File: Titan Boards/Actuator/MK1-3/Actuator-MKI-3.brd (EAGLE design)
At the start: 101.6 x 55.9 mm, 56 parts, among them U1 DRV8816PWPR, U2 MBRB2060CTT4G, U3 MBRB2060CTT4G, U4 MBRB2060CTT4G, U5 MBRB2060CTT4G, U6 MBRB2060CTT4G, U7 MBRB2060CTT4G

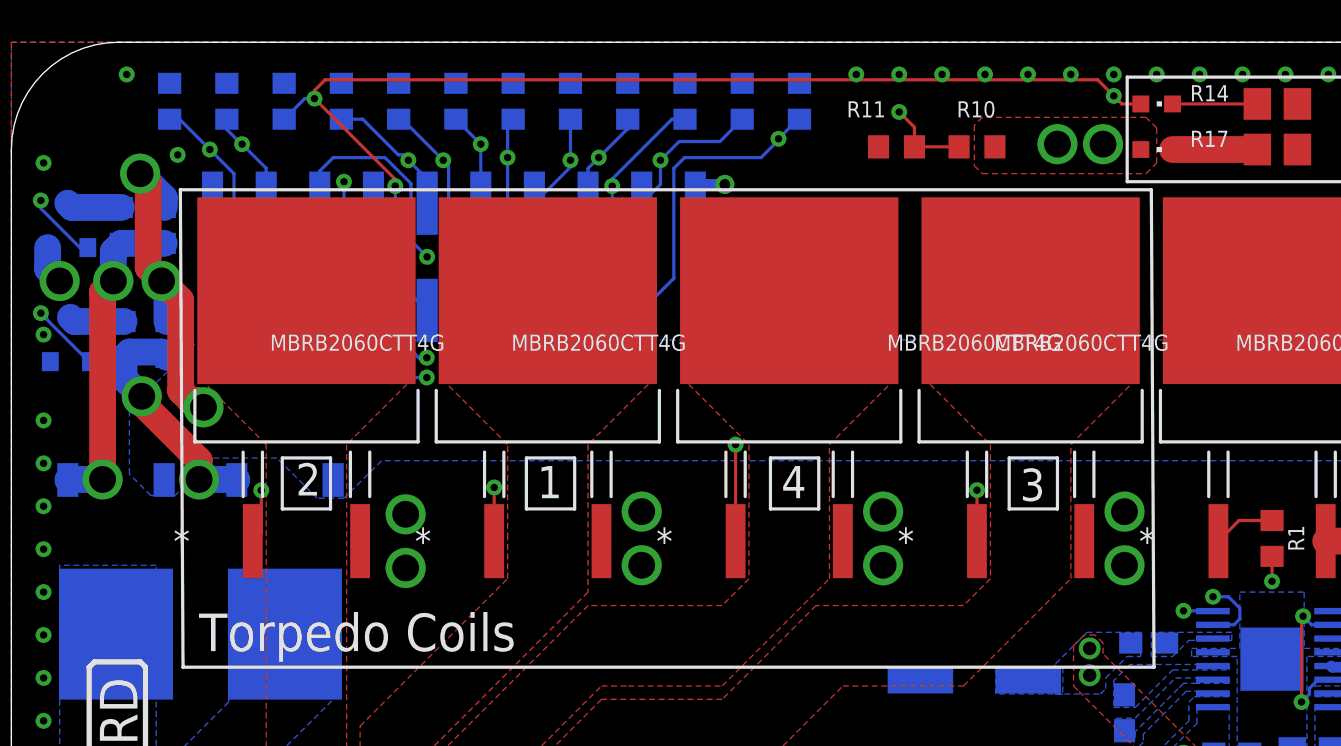
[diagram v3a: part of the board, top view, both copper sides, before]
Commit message: Tempest Actuator Updates
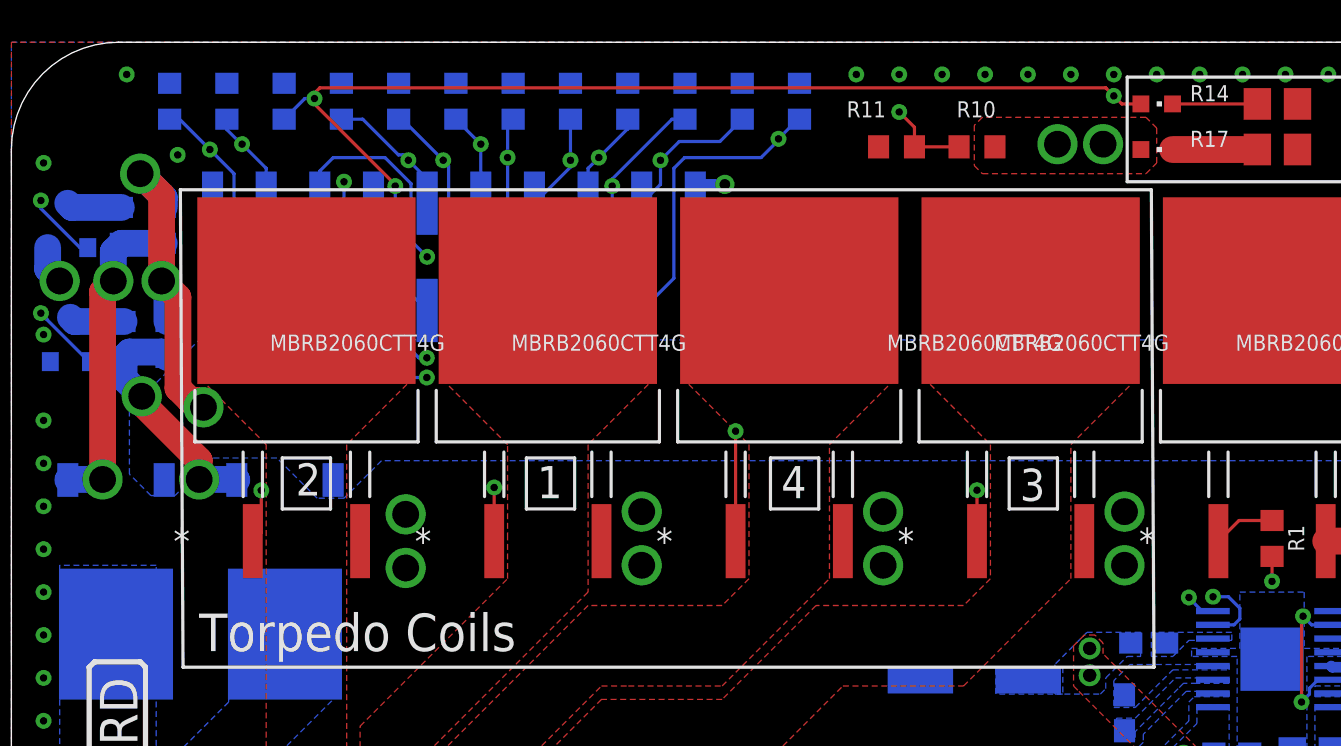
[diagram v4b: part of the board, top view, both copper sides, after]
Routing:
- net PWM_DRIVER1: track 77.5 -> 80.4 mm
- net VPROPI: track 59.1 -> 59.8 mm

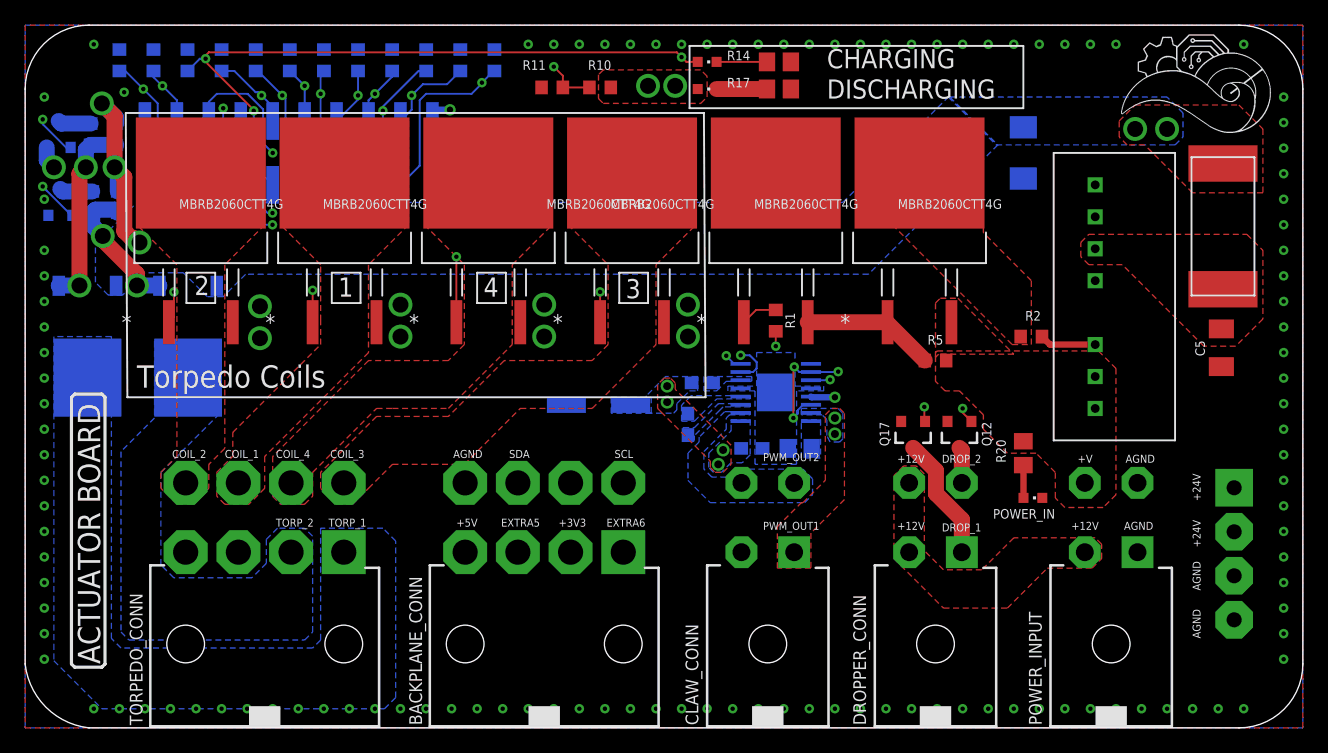
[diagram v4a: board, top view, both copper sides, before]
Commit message: Tempest Actuator Board Review Revisions
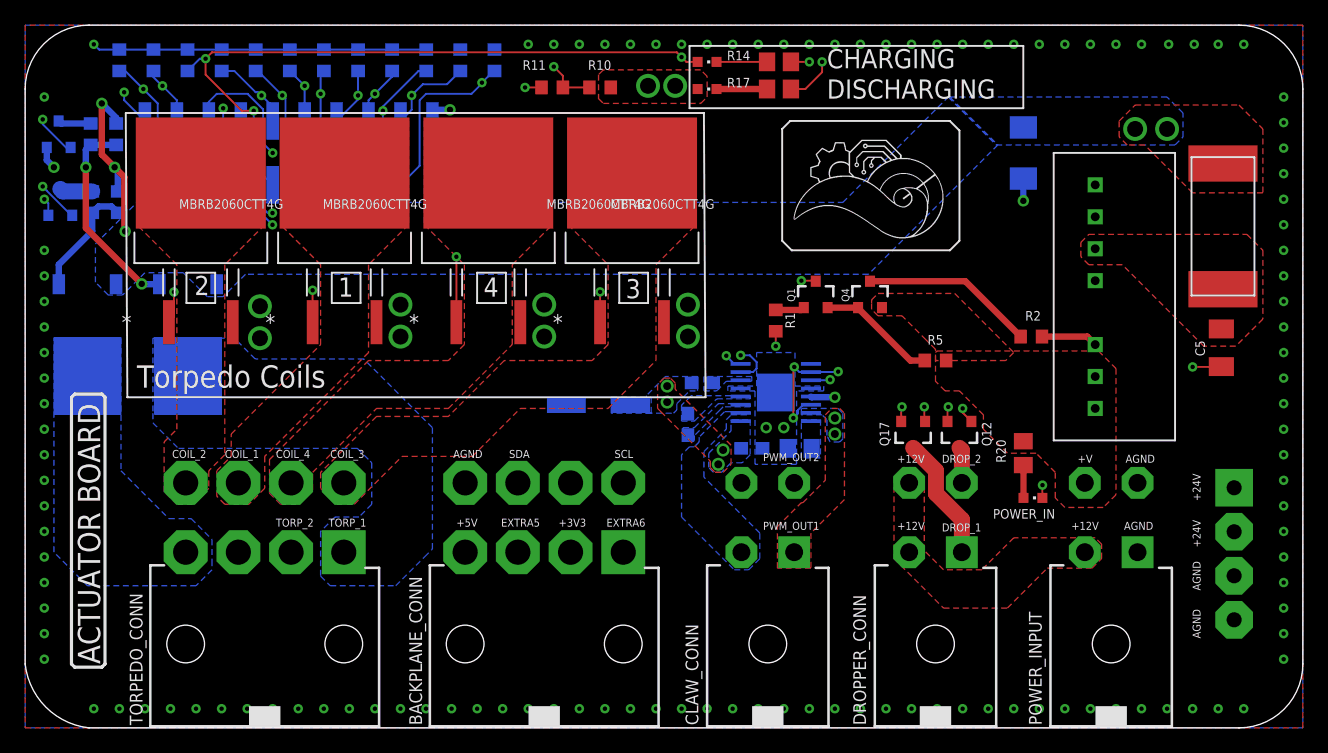
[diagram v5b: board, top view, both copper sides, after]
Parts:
- removed U6, U7: MBRB2060CTT4G, DPAK2:D2PAK3-4_9P65X10P29_ONS
- added Q1, Q4: (no value), SparkFun-DiscreteSemi:SOT23-3
- moved Q18 8.00 mm to (13.0, 30.5)
- moved Q6 8.00 mm to (4.95, 30.5)
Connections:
- removed net EXTRA5: BACKPLANE_CONN.3
- removed net EXTRA6: BACKPLANE_CONN.1
- net +3V3: now also BACKPLANE_CONN.1; no longer BACKPLANE_CONN.2
- net AGND: now also Q1.3; no longer U7.4
- net N$5: now also Q1.1; no longer U7.3
- net N$6: now also Q1.2, Q4.1; no longer U6.3, U7.1
- net N$7: now also Q4.3; no longer U6.4
- net PWM_OUT2: now also CLAW_CONN.2; no longer CLAW_CONN.3
- net TORPEDO2: now also TORPEDO_CONN.4; no longer TORPEDO_CONN.2
- net V+: now also Q4.2; no longer U6.1
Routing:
- net AGND: track 1.82 -> 53.1 mm, vias 124 -> 139
- net N$7: track 0.00 -> 13.8 mm
- net DROPPER2_GATE: track 76.5 -> 66.4 mm
- net DROPPER1_GATE: track 80.3 -> 70.3 mm
- net +3V3: track 81.1 -> 77.1 mm
- net V_DIV: track 40.9 -> 38.4 mm
- net N$35: track 11.3 -> 9.23 mm, vias 2 -> 0
- net +24V: track 16.6 -> 15.1 mm
- net N$33: track 15.2 -> 16.5 mm
- net N$6: track 10.7 -> 9.49 mm
- net N$5: track 2.94 -> 2.30 mm
- removed copper zone on layer 1, net N$7
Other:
- board text added: "COIL1 GATE"
- board text added: "COIL3 GATE"
- board text added: "DROP2 GATE"
- board text added: "TORP2 GATE"
